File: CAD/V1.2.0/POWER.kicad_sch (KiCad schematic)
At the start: 52 parts, among them K1 Inkplate_TP, U1 TPS65186RGZ

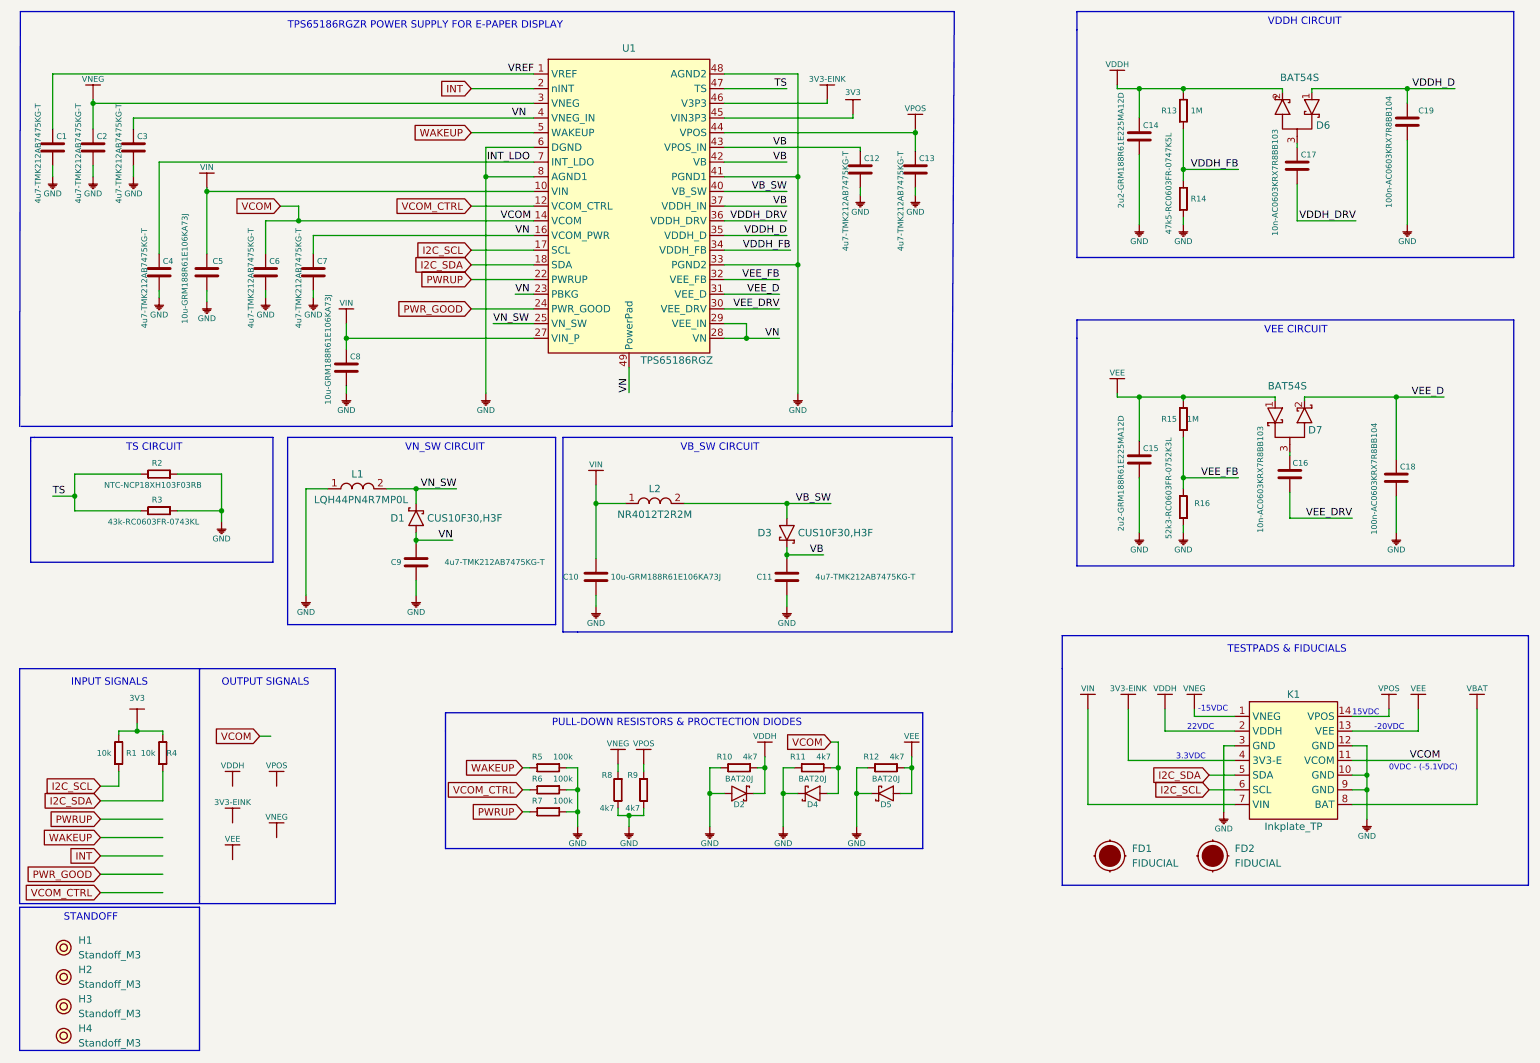
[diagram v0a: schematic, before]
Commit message: Updating open source files.
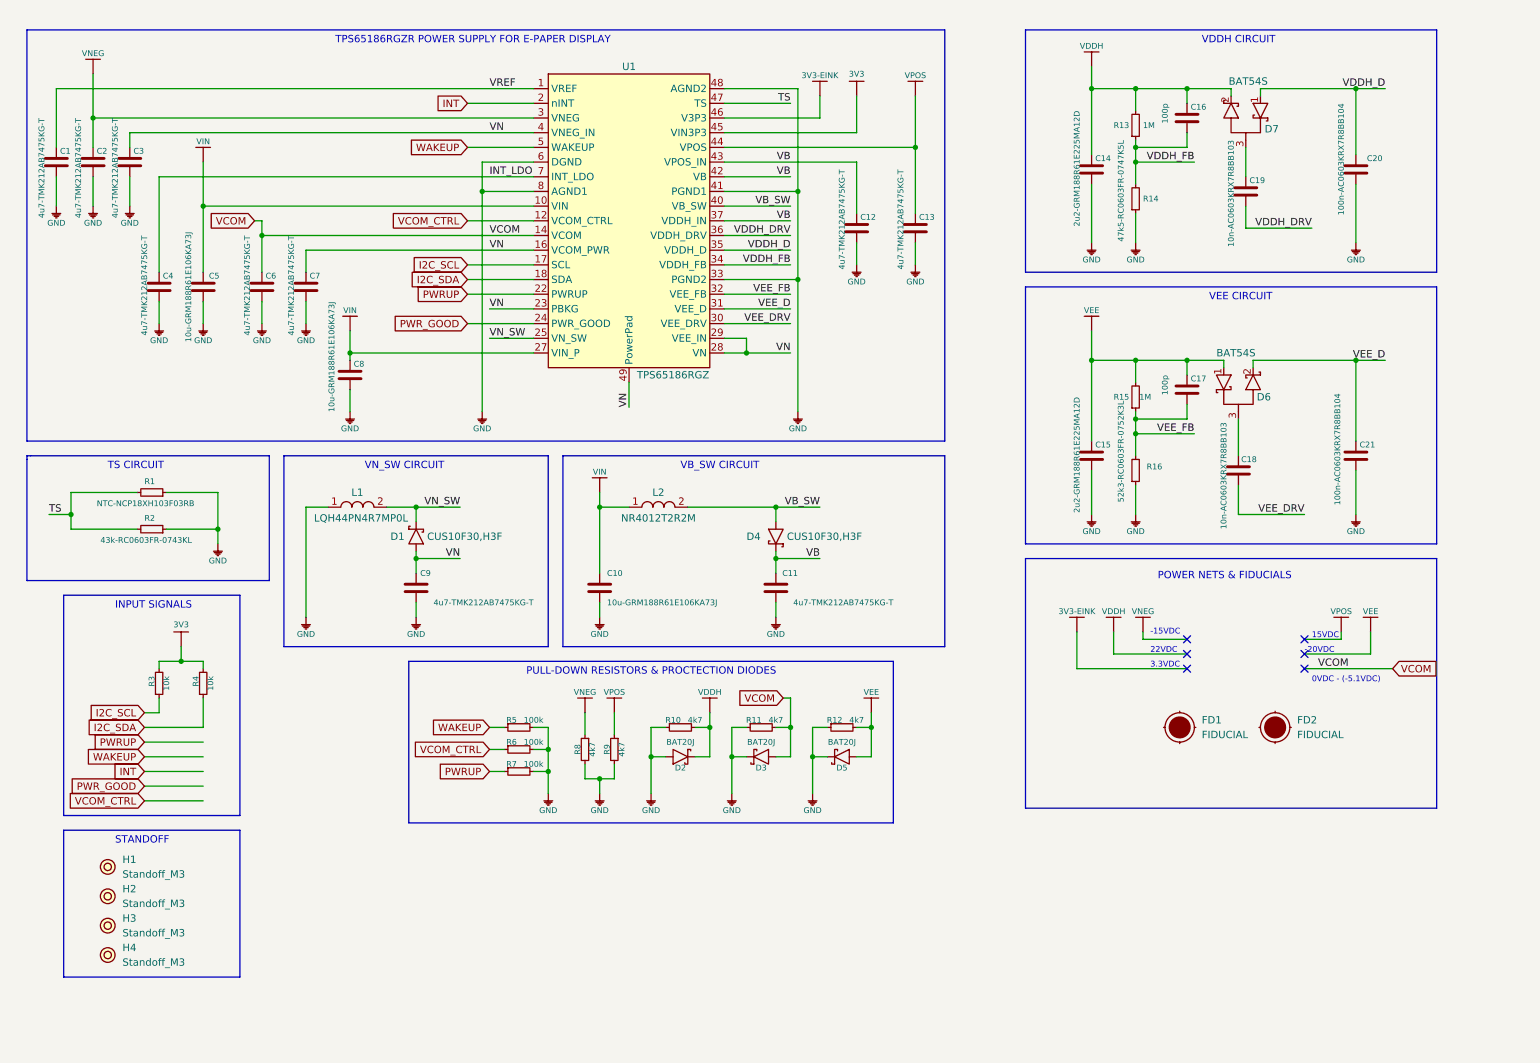
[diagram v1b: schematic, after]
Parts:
- removed K1: Inkplate_TP, e-radionica.com footprinti:INKPLATE TEST HEADER, symbol e-radionica.com schematics:Inkplate_TP
- added C16, C17: 100p, e-radionica.com footprinti:0603C, symbol e-radionica.com schematics:0603C
- renumbered C16 to C18, C17 to C19, C19 to C20, C18 to C21, D4 to D3, D3 to D4, D7 to D6, D6 to D7, R2 to R1, R3 to R2, R1 to R3
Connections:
- net VDDH: now also C16.2
- net VDDH_FB: now also C16.1
- net VEE: now also C17.2
- net VEE_FB: now also C17.1
- no-connect marks 0 -> 6
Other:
- note added: "POWER NETS & FIDUCIALS"
- note removed: "OUTPUT SIGNALS"
- note removed: "TESTPADS & FIDUCIALS"
- title: Soldered Inkplate 6PLUS -> Soldered Inkplate 6 FLICK
- moved on the sheet: C1, C10, C11, C12, C13, C14, C15, C18, C19, C2, C20, C21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
